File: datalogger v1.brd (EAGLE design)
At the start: 102.9 x 58.6 mm, 19 parts, among them M2 ARDUINO-NANO-3.0

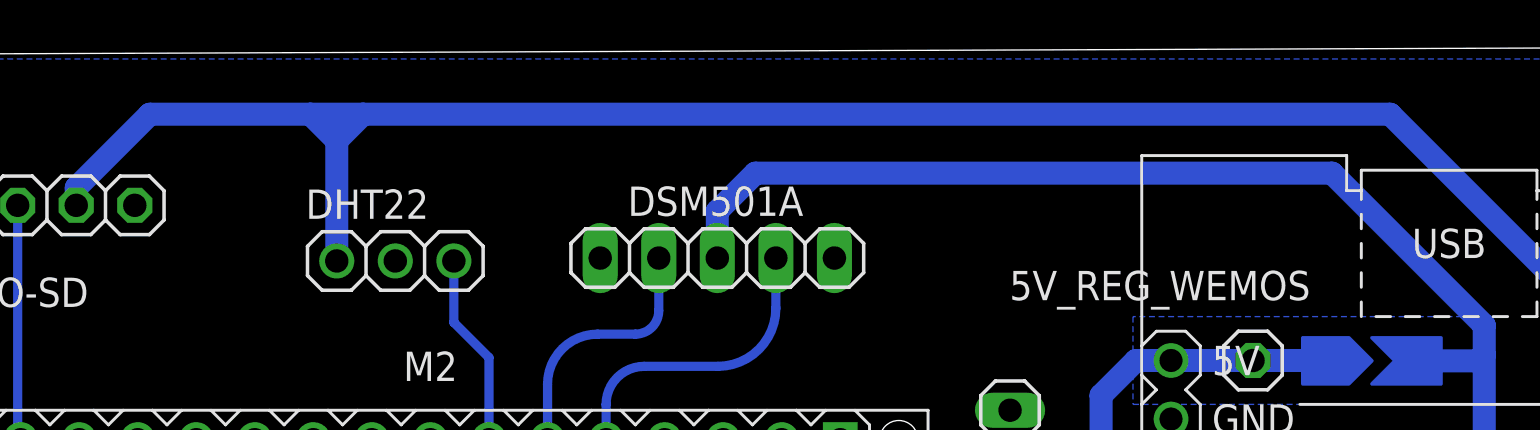
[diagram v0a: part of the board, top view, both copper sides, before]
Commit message: update pcb
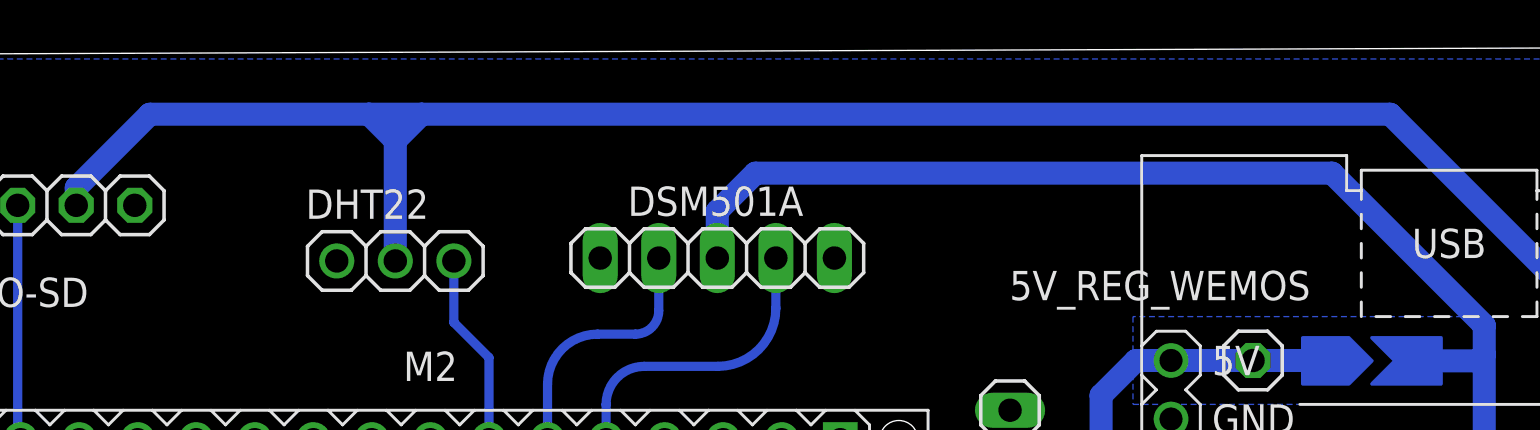
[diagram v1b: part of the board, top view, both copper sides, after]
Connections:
- net 5V: now also DHT22.2; no longer DHT22.1
- net GND: now also DHT22.1; no longer DHT22.2
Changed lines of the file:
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@@
 <signals>
 <signal name="5V">
-<contactref element="DHT22" pad="1"/>
 <contactref element="RTC" pad="2"/>
 <contactref element="MICRO-SD" pad="2"/>
@@
 <wire x1="11.938" y1="4.826" x2="13.208" y2="3.556" width="1" layer="16"/>
 <wire x1="13.208" y1="3.556" x2="16.637" y2="3.556" width="1" layer="16"/>
-<wire x1="78.4686" y1="56.1514" x2="33.909" y2="56.1514" width="1" layer="16"/>
+<wire x1="78.4686" y1="56.1514" x2="36.449" y2="56.1514" width="1" layer="16"/>
+<wire x1="36.449" y1="56.1514" x2="34.163" y2="56.1514" width="1" layer="16"/>
 <contactref element="M2" pad="J2.4"/>
-<wire x1="33.909" y1="56.1514" x2="31.623" y2="56.1514" width="1" layer="16"/>
-<wire x1="31.623" y1="56.1514" x2="24.6554" y2="56.1514" width="1" layer="16"/>
+<wire x1="34.163" y1="56.1514" x2="24.6554" y2="56.1514" width="1" layer="16"/>
 <wire x1="46.99" y1="26.797" x2="46.99" y2="26.416" width="1" layer="16"/>
 <wire x1="24.6554" y1="56.1514" x2="21.463" y2="52.959" width="1" layer="16"/>
@@
 <wire x1="50.927" y1="53.594" x2="49.276" y2="51.943" width="1" layer="16"/>
 <wire x1="49.276" y1="51.943" x2="49.276" y2="49.911" width="1" layer="16"/>
-<wire x1="31.623" y1="56.1514" x2="32.766" y2="55.0084" width="1" layer="16"/>
+<wire x1="34.163" y1="56.1514" x2="35.306" y2="55.0084" width="1" layer="16"/>
 <wire x1="39.3065" y1="4.7625" x2="39.37" y2="4.699" width="1" layer="16"/>
 <wire x1="39.37" y1="4.699" x2="40.513" y2="3.556" width="1" layer="16"/>
@@
 <wire x1="18.034" y1="7.493" x2="18.034" y2="3.937" width="1" layer="16"/>
 <wire x1="18.034" y1="3.937" x2="17.653" y2="3.556" width="1" layer="16"/>
-<wire x1="33.909" y1="56.1514" x2="32.766" y2="55.0084" width="1" layer="16"/>
-<wire x1="32.766" y1="55.0084" x2="32.766" y2="49.784" width="1" layer="16"/>
+<wire x1="36.449" y1="56.1514" x2="35.306" y2="55.0084" width="1" layer="16"/>
 <contactref element="U$4" pad="J2"/>
 <contactref element="U$5" pad="J2"/>
@@
 <wire x1="28.305" y1="5.795" x2="28.305" y2="3.921" width="1" layer="16"/>
 <wire x1="28.305" y1="3.921" x2="27.94" y2="3.556" width="1" layer="16"/>
+<contactref element="DHT22" pad="2"/>
+<wire x1="35.306" y1="55.0084" x2="35.306" y2="49.784" width="1" layer="16"/>
 <wire x1="46.99" y1="26.797" x2="49.276" y2="49.911" width="0" layer="19" extent="1-1"/>
 </signal>
@@
 <wire x1="81.989" y1="2.926" x2="75.443" y2="2.926" width="1" layer="16"/>
 <wire x1="75.443" y1="2.926" x2="75.438" y2="2.921" width="1" layer="16"/>
-<contactref element="DHT22" pad="2"/>
+<contactref element="DHT22" pad="1"/>
 </signal>
 <signal name="SDA">

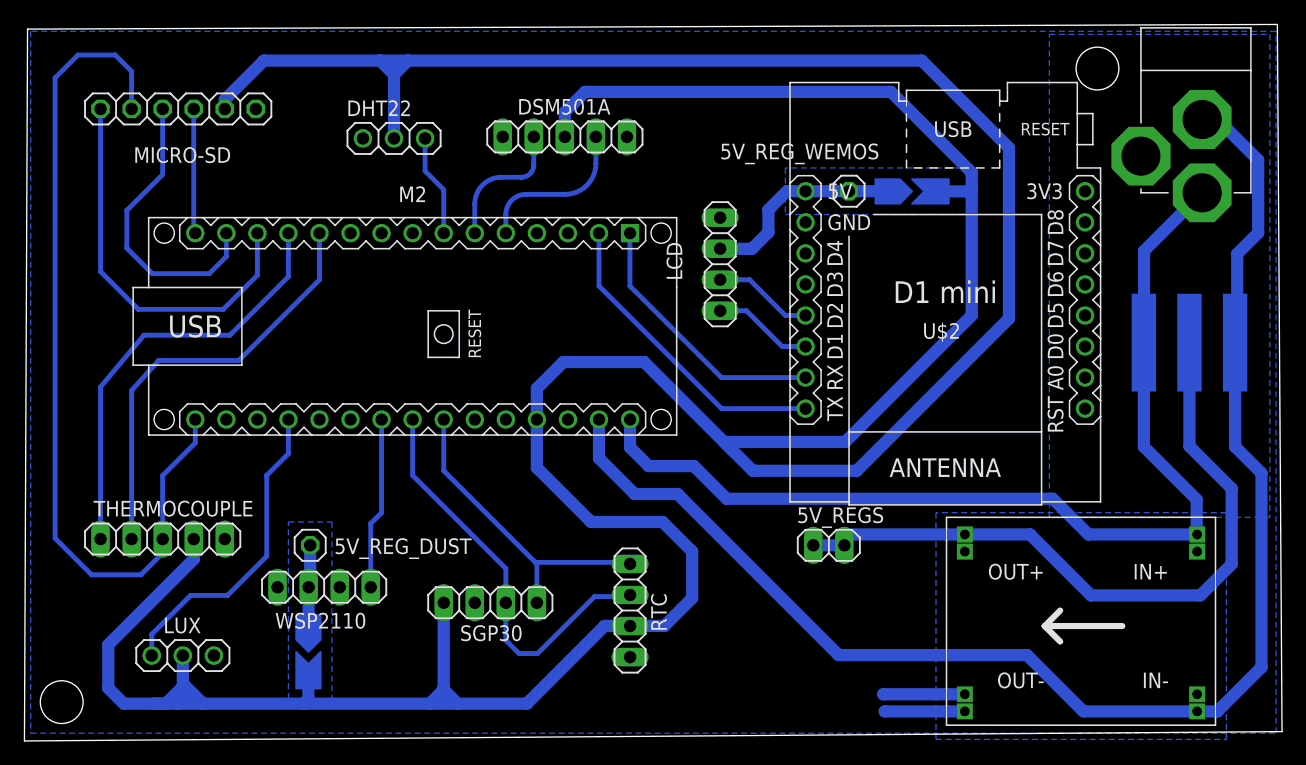
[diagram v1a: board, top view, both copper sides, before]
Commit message: update
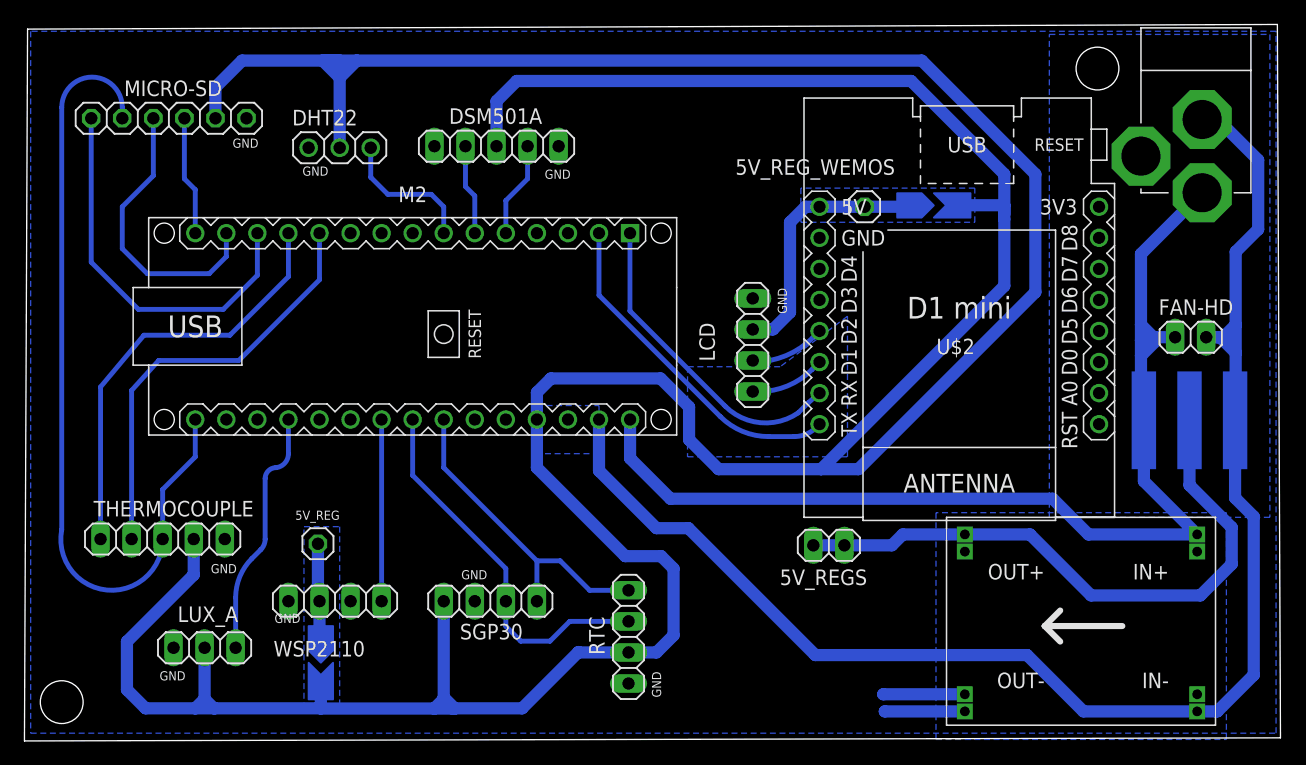
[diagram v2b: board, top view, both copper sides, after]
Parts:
- removed 5V_REG_DUST: (no value), pinhead:1X01
- removed LUX: (no value), adafruit:1X03
- removed U$4, U$5: JUMP-NO, P_Dusk:JOMP-NO
- added 5V_REG: (no value), pinhead:1X01
- added FAN-HD: (no value), pinhead:1X02
- added LUX_A: (no value), pinhead:1X03
- added NO-JUMP-PAD2, NO-JUMP_PAD: JUMP-NO, P_Dusk:JOMP-NO
- moved LCD 7.12 mm to (64.6, 32.9)
- moved U$3 6.35 mm to (95.6, 22.7)
- moved DSM501A 5.64 mm to (43.7, 49.1)
- moved DHT22 4.51 mm to (30.9, 49.0)
- moved RTC 2.16 mm to (54.5, 9.02)
- moved 5V_REG_WEMOS 1.80 mm to (73.8, 44.2)
- moved U$2 1.71 mm to (81.5, 35.9)
- moved WSP2110 1.45 mm to (30.5, 11.9)
- moved MICRO-SD 1.08 mm to (16.9, 51.4)
- moved SGP30 0.13 mm to (43.2, 11.9)
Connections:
- removed net N$1: DSM501A.1
- net 12V: now also FAN-HD.1
- net 5V: now also LUX_A.2, NO-JUMP-PAD2.J2, NO-JUMP_PAD.J2; no longer LUX.2, U$4.J2, U$5.J2
- net 5V_REG: now also 5V_REG.1, NO-JUMP-PAD2.J1; no longer 5V_REG_DUST.1, U$5.J1
- net GND: now also LUX_A.3; no longer LUX.3
- net GND_ADP: now also FAN-HD.2
- net LUX_A: now also LUX_A.1; no longer LUX.1
- net N$2: now also NO-JUMP_PAD.J1; no longer U$4.J1
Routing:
- net CLK: track 71.1 -> 60.9 mm
- net 12V: track 83.6 -> 91.4 mm
- net 5V: track 334.5 -> 341.2 mm
- net LUX_A: track 25.7 -> 20.1 mm
- net VOUT-1: track 12.8 -> 7.85 mm
- net 5V_REG: track 63.7 -> 58.9 mm
- net N$2: track 16.7 -> 21.3 mm
- net RX_WEMOS: track 21.8 -> 25.8 mm
- net GND_ADP: track 116.1 -> 119.8 mm
- net VOUT-2: track 11.0 -> 7.61 mm
- net DATA-DHT22: track 8.38 -> 11.5 mm
- net SDA: track 33.9 -> 31.4 mm
- net TX_WEMOS: track 25.4 -> 27.8 mm
- net SCL_LCD: track 8.19 -> 6.07 mm
- net SDA_LCD: track 8.19 -> 6.13 mm
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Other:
- board size 102.9 x 58.6 mm -> 102.7 x 58.6 mm
- board text added: "GND"
